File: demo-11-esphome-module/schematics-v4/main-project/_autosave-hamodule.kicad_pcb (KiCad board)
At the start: 2 copper layers, 165.1 x 67.3 mm, 54 parts, among them J1 1017505, J2 1017505, J4 1017505, K1 G5Q-1, K2 G5Q-1, K3 G5Q-1, K4 G5Q-1, Q1 2N2219, Q2 2N2219, Q3 2N2219, Q4 2N2219, U1 ESP32-DEVKITC-32D, U2 HCPL3700, U3 HCPL3700, U4 HCPL3700, U5 HCPL3700

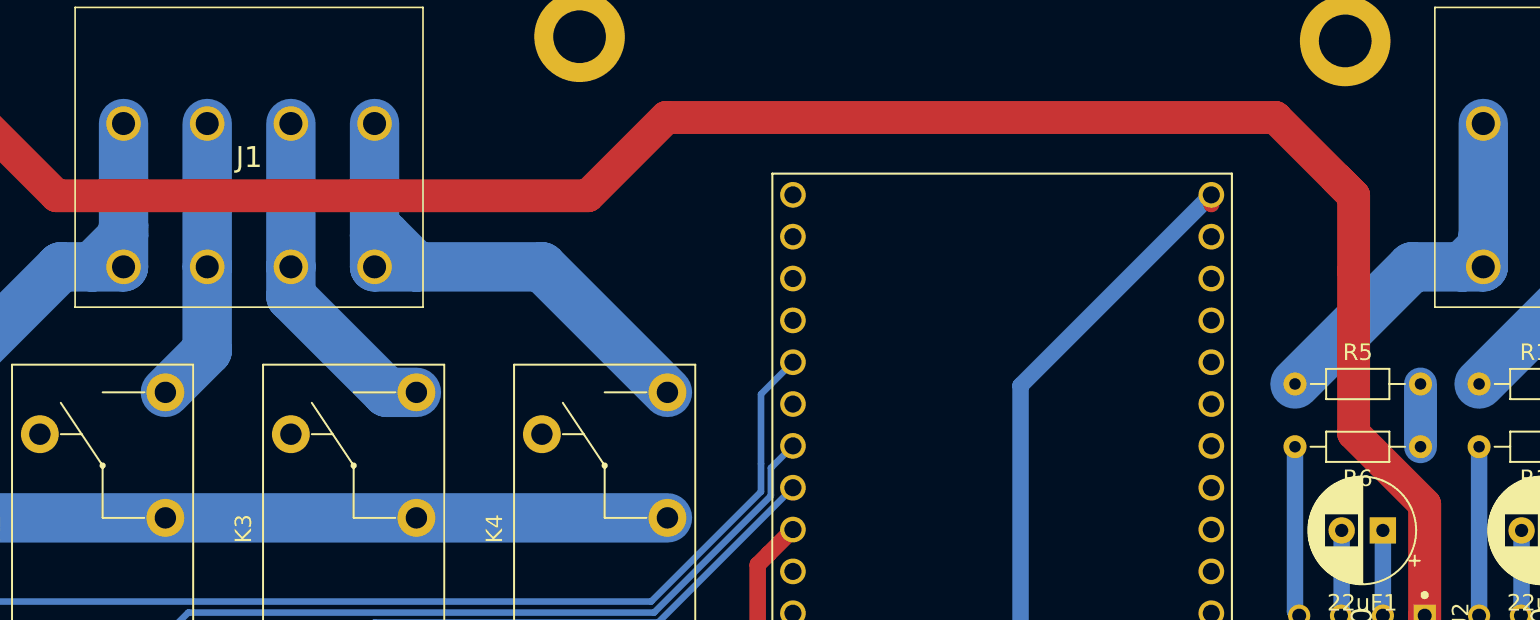
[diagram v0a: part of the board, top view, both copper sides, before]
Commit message: some changes to schema
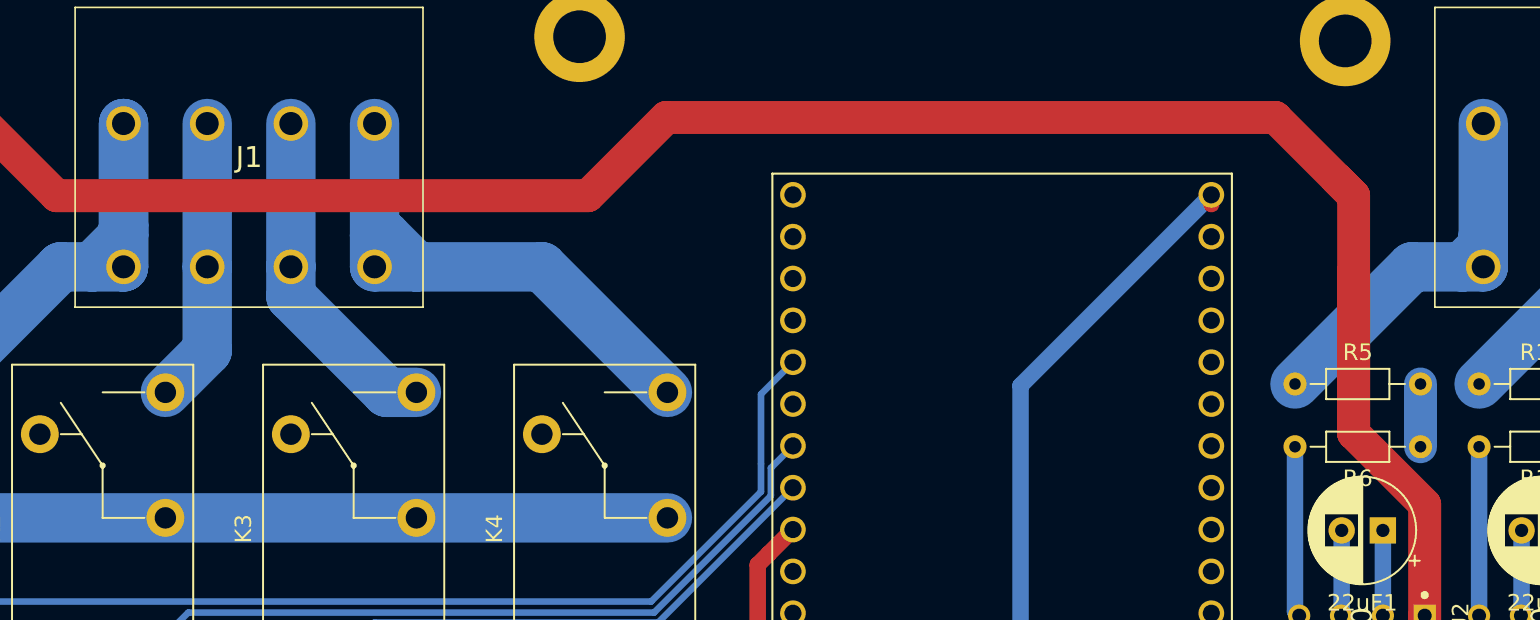
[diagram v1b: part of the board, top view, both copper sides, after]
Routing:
- net 220VAC(N): track 205.8 -> 215.7 mm
- net REO1: track 26.6 -> 35.3 mm
